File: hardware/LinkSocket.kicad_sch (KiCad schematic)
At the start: 4 parts, among them J2001 2x05_Horizontal, U2001 THVD24x2

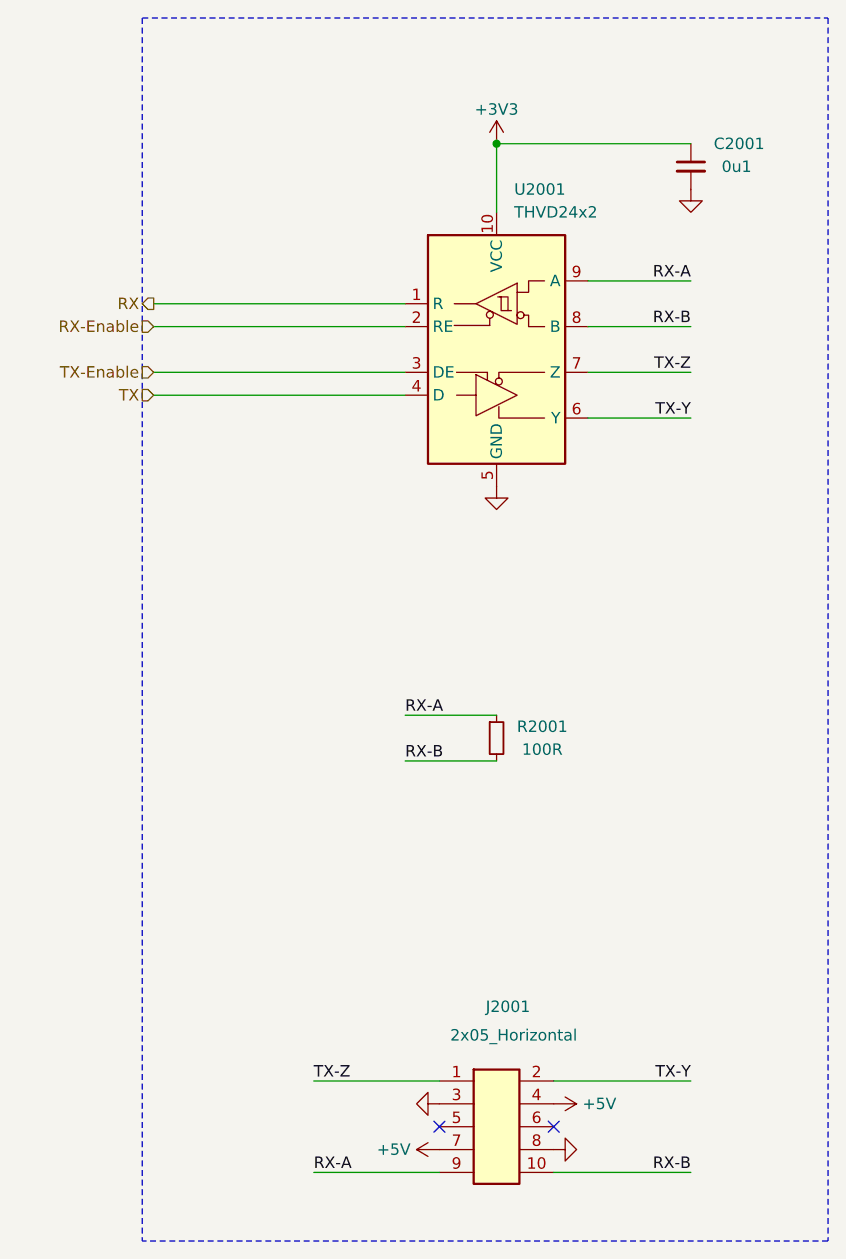
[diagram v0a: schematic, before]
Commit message: Update parts library
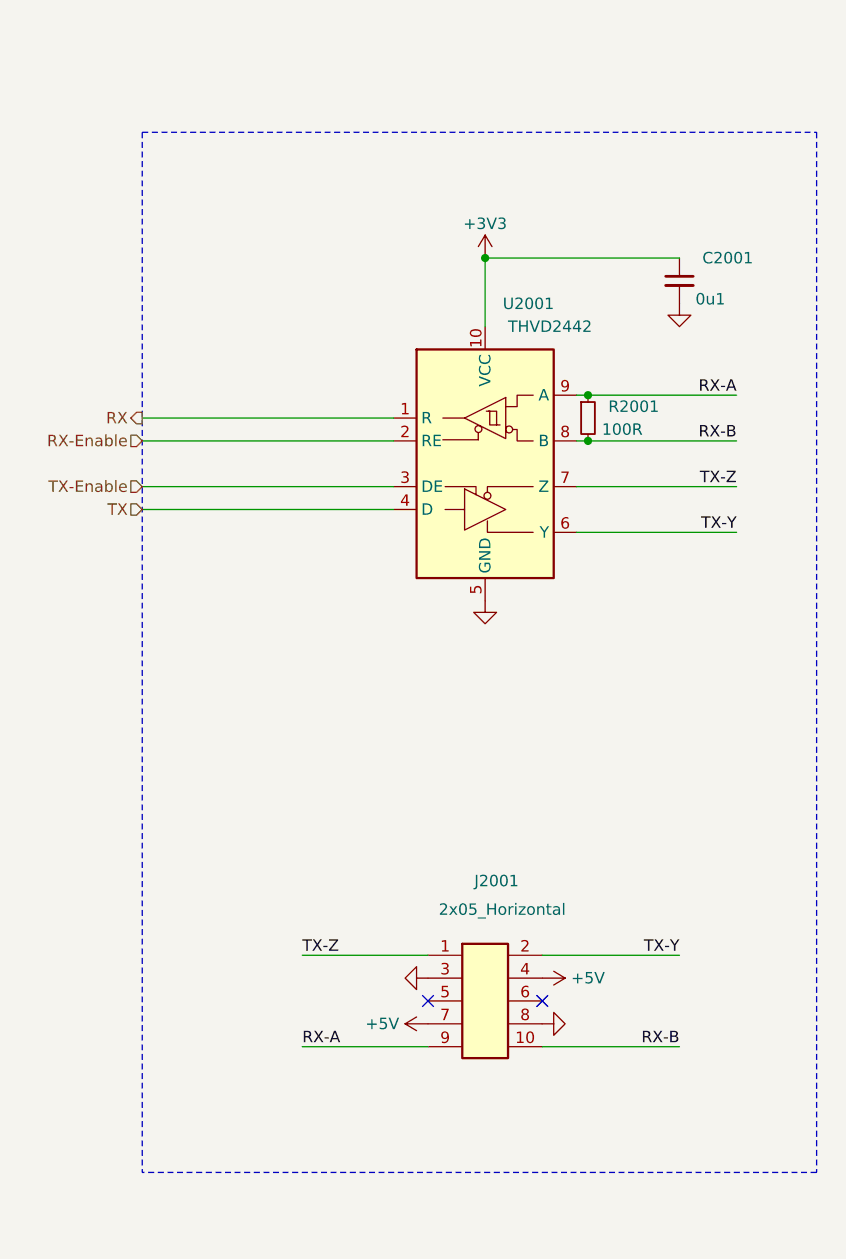
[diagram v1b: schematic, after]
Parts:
- C2001: footprint Capacitor_SMD:C_0603_1608Metric -> V2_Capacitor_SMD:C_0603; symbol Device:C_Small -> V2_Device:C_0603_0u1; Mouser (none) -> 810-CGA3E2X7R1H104MA
- J2001: Mouser (none) -> 649-200211120001T4LF
- R2001: footprint Resistor_SMD:R_0603_1608Metric -> V2_Resistor_SMD:R_0603; symbol Device:R_Small -> V2_Device:R_0603_100R; Mouser (none) -> 71-CRCW0603100RFKEAH
- U2001: value THVD24x2 -> THVD2442; symbol V2_Interface_RS485:THVD24x2 -> V2_Interface_RS485:THVD2442; Mouser (none) -> 595-THVD2442DRCR
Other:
- moved on the sheet: C2001, J2001, R2001, U2001
